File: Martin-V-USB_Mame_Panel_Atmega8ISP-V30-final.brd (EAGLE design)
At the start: 50 x 50 mm, 22 parts, among them IC1 MEGA8-P, IC2 LD117ADT33TR, Q1 12MHz, X1 USB

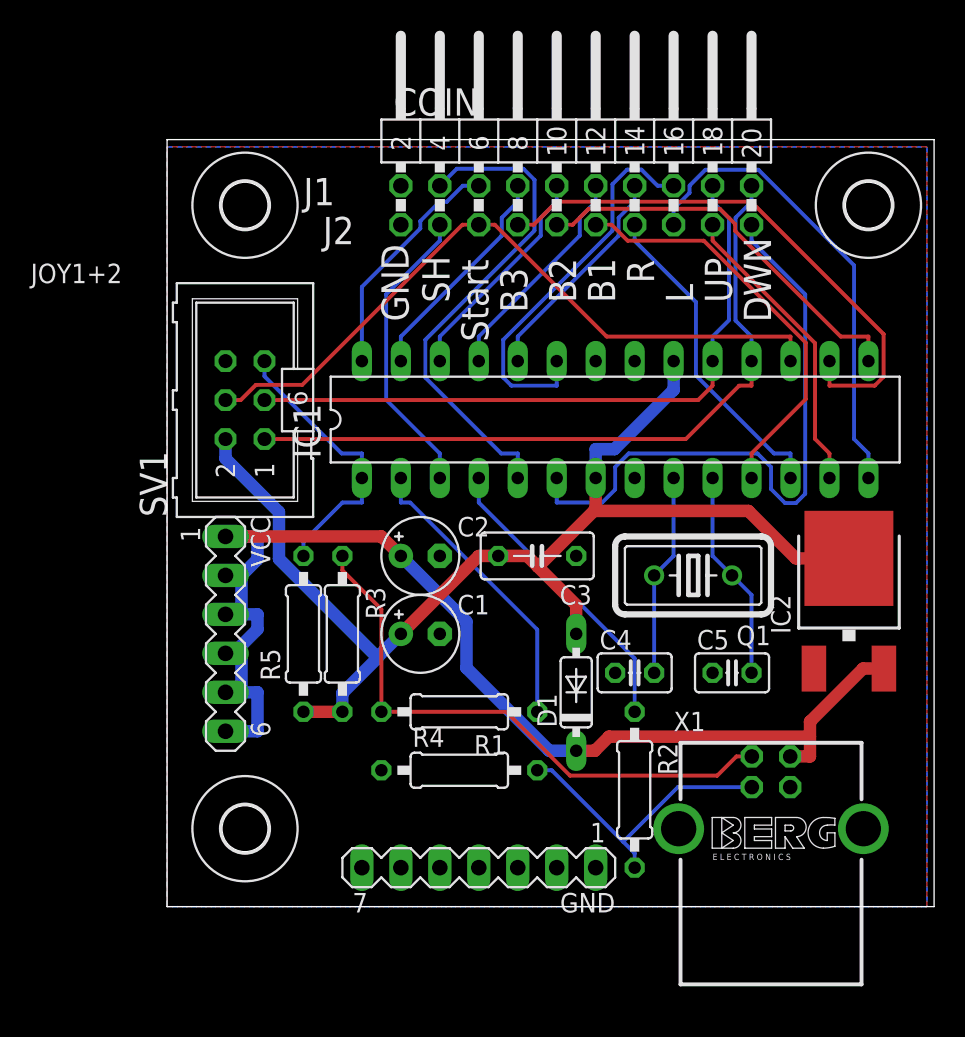
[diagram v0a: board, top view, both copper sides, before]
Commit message: v3
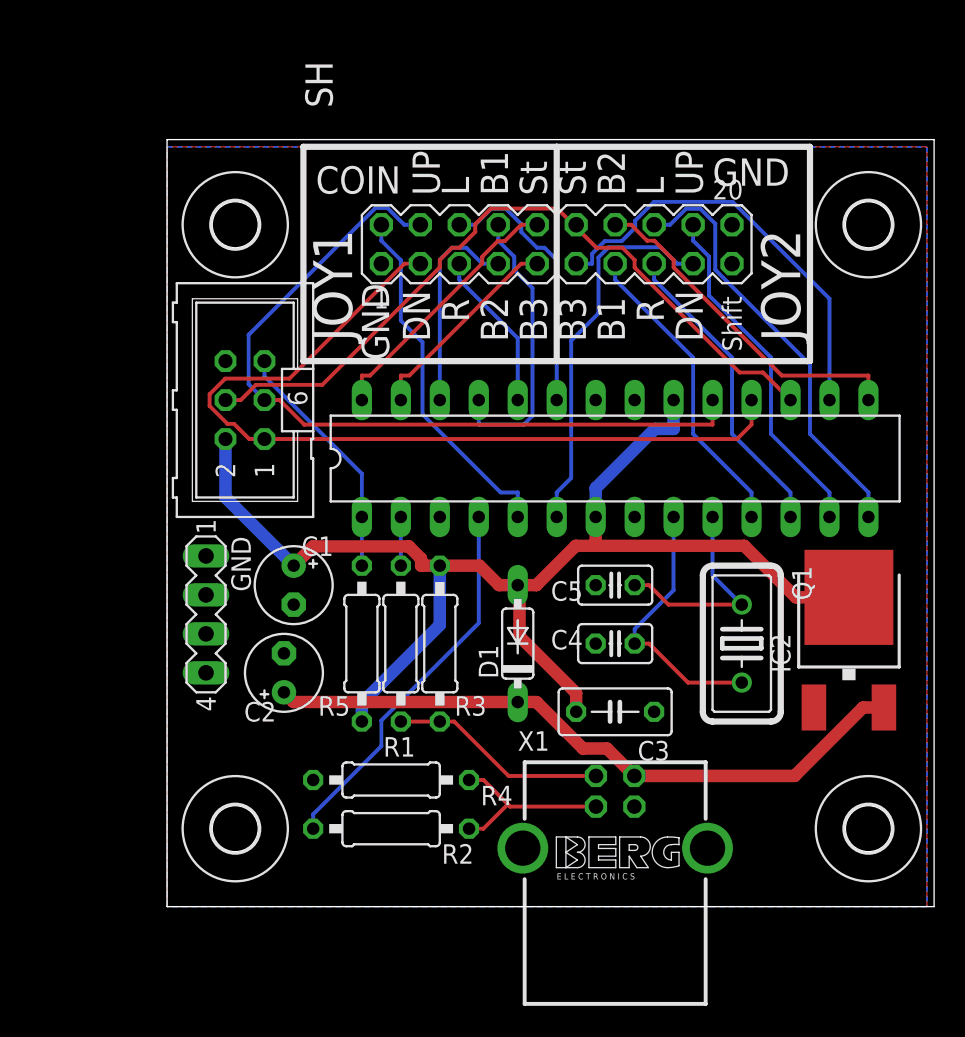
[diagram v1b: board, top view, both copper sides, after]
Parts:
- removed VCC: (no value), con-lstb:MA06-1
- added U$4: (no value), holes:3,0
- GND: device con-lstb:MA07-1 -> con-lstb:MA04-1
- JOY1+2: device con-lstb:MA10-2W -> con-lstb:MA10-2
- moved GND 24.3 mm to (2.54, 19.1), turned to 270 degrees
- moved R2 16.1 mm to (14.6, 5.08), turned to 0 degrees
- moved C2 11.7 mm to (7.62, 15.2), turned to 90 degrees
- moved C3 11.4 mm to (29.2, 12.7)
- moved X1 10.2 mm to (29.2, 3.81)
- moved C5 9.52 mm to (29.2, 21.0)
- moved C1 8.84 mm to (8.26, 21.0), turned to 270 degrees
- moved R3 6.38 mm to (17.8, 17.1), turned to 90 degrees
- moved R1 5.85 mm to (15.2, 17.1), turned to 270 degrees
- moved Q1 5.46 mm to (37.5, 17.1), turned to 270 degrees
- moved D1 4.96 mm to (22.9, 17.1)
- moved R4 4.49 mm to (14.6, 8.26)
- moved R5 3.86 mm to (12.7, 17.1)
- moved JOY1+2 2.84 mm to (25.4, 43.2)
- moved IC1 2.54 mm to (29.2, 29.2)
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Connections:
- net +5V: no longer VCC.1, VCC.2, VCC.3, VCC.4, VCC.5, VCC.6
- net COINTRIGGER: now also JOY1+2.2; no longer JOY1+2.4
- net GND: now also JOY1+2.20; no longer GND.5, GND.6, GND.7, JOY1+2.2
- net JOY1BUTTON1: now also JOY1+2.8; no longer JOY1+2.12
- net JOY1BUTTON2: now also JOY1+2.7; no longer JOY1+2.10
- net JOY1BUTTON3: now also JOY1+2.9; no longer JOY1+2.8
- net JOY1DOWN: now also JOY1+2.3; no longer JOY1+2.20
- net JOY1LEFT: now also JOY1+2.6; no longer JOY1+2.16
- net JOY1RIGHT: now also JOY1+2.5; no longer JOY1+2.14
- net JOY1START: now also JOY1+2.10; no longer JOY1+2.6
- net JOY1UP: now also JOY1+2.4; no longer JOY1+2.18
- net JOY2BUTTON1: now also JOY1+2.13; no longer JOY1+2.11
- net JOY2BUTTON2: now also JOY1+2.14; no longer JOY1+2.9
- net JOY2BUTTON3: now also JOY1+2.11; no longer JOY1+2.7
- net JOY2DOWN: now also JOY1+2.17; no longer JOY1+2.19
- net JOY2LEFT: now also JOY1+2.16; no longer JOY1+2.15
- net JOY2RIGHT: now also JOY1+2.15; no longer JOY1+2.13
- net JOY2START: now also JOY1+2.12; no longer JOY1+2.5
- net JOY2UP: now also JOY1+2.18; no longer JOY1+2.17
- net SHIFTSWITCH: now also JOY1+2.19; no longer JOY1+2.3
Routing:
- net +5V: track 80.0 -> 43.2 mm
- net N$4: track 37.6 -> 14.2 mm
- net SHIFTSWITCH: track 19.4 -> 0.00 mm
- net JOY2DOWN: track 41.4 -> 24.9 mm
- net N$1: track 19.3 -> 3.17 mm
- net JOY1DOWN: track 47.1 -> 56.2 mm
- net COINTRIGGER: track 32.4 -> 23.4 mm
- net JOY2BUTTON3: track 36.2 -> 28.1 mm
- net JOY1LEFT: track 25.7 -> 17.6 mm
- net JOY1UP: track 43.5 -> 51.2 mm
- net N$5: track 19.4 -> 12.2 mm
- net JOY2BUTTON1: track 27.2 -> 20.2 mm
- net N$2: track 19.4 -> 24.8 mm
- net +3V3: track 79.9 -> 84.9 mm
- net JOY1BUTTON1: track 14.6 -> 18.7 mm
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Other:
- board text added: "DN"
- board text added: "JOY1"
- board text added: "JOY2"
- board text added: "Shift"
- board text added: "St"
- board text added: "VUSB-MAME V3.0 www.neuby.de"
- board text removed: "DWN"
- board text removed: "J1"
- board text removed: "J2"
- board text removed: "Start"
